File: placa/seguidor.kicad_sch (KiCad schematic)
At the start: 17 parts, among them J1 Conn_01x02_Pin, J2 Conn_01x15_Socket, SW1 btn_reset, SW2 btn_arranque, U1 ATmega328P-P, U2 LM7805_TO220, Y1 Crystal

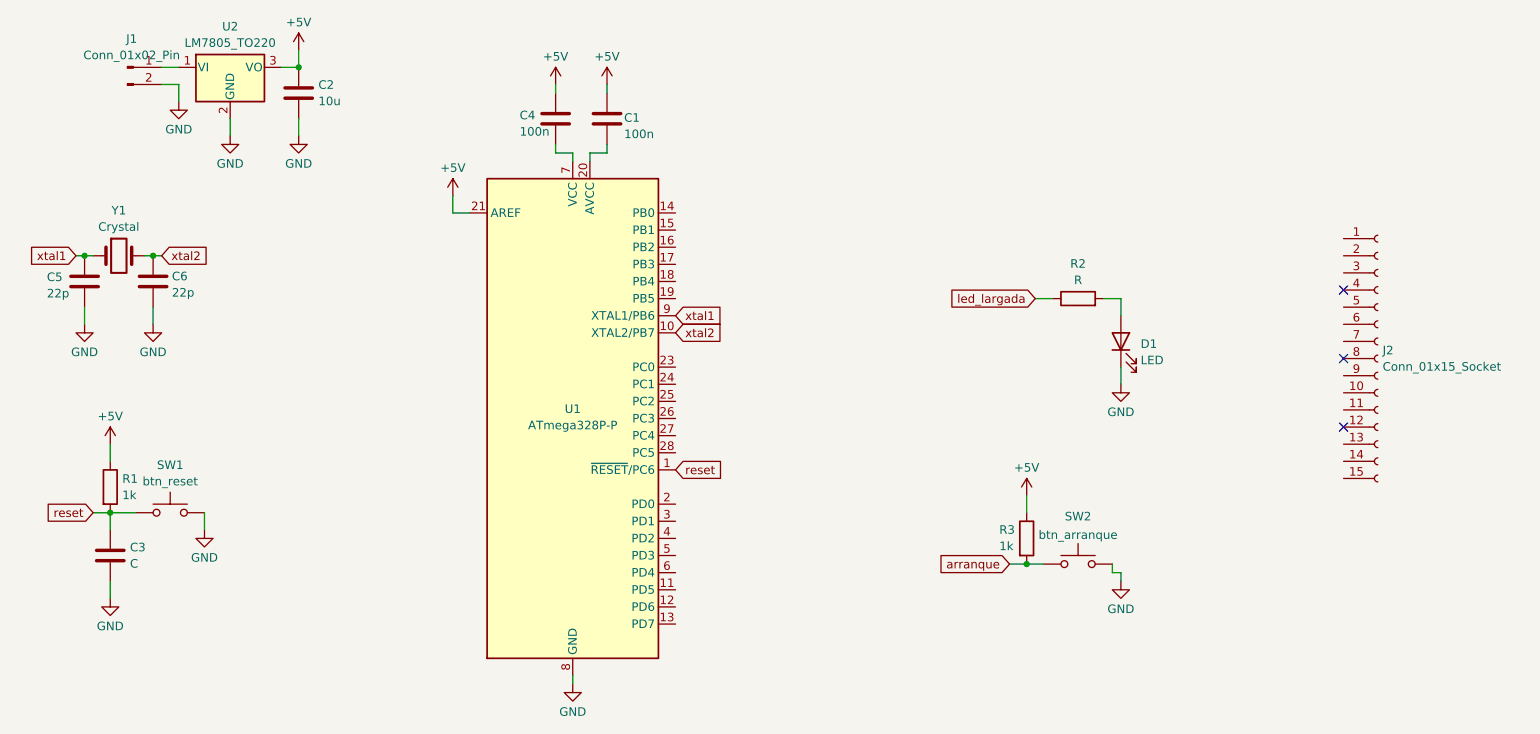
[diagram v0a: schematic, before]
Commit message: circuito modificado
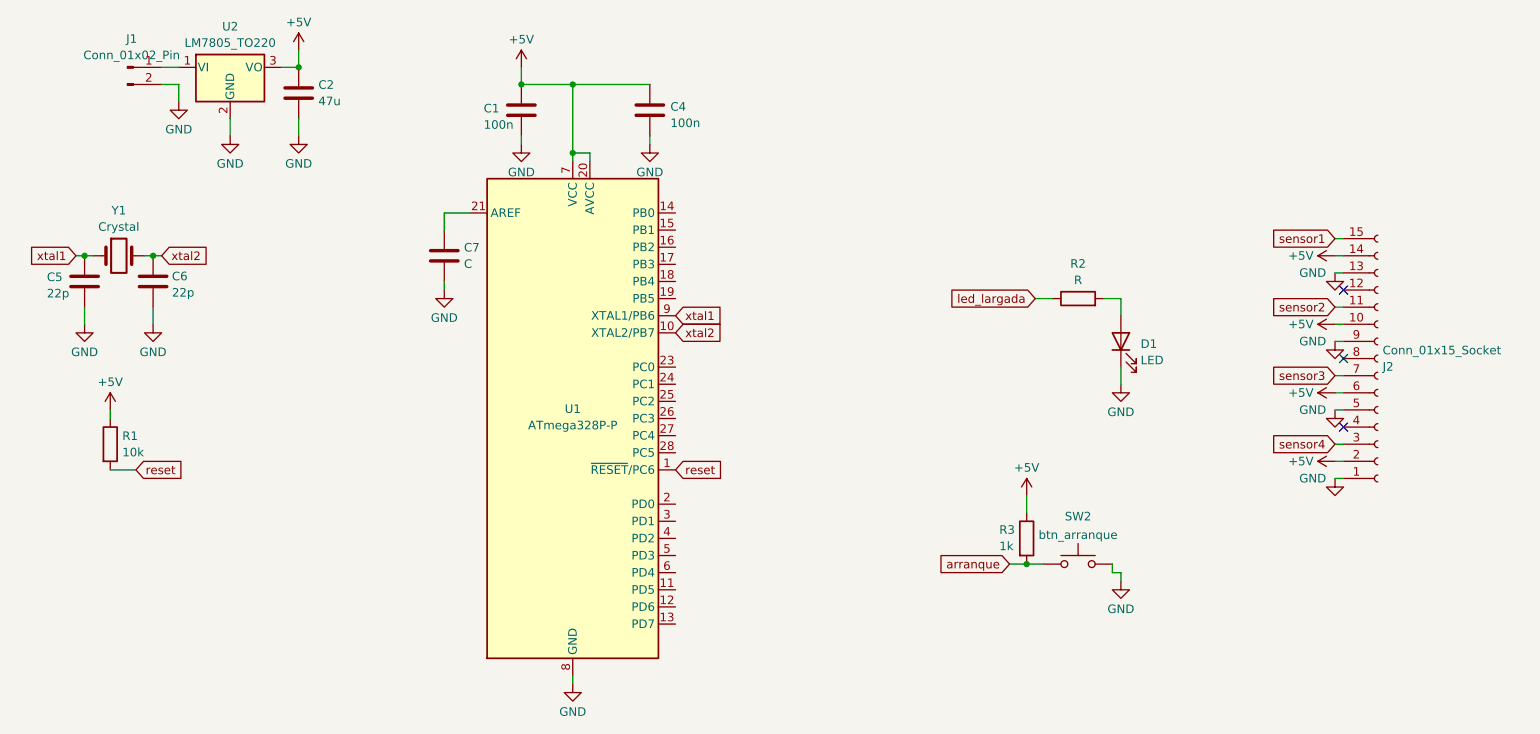
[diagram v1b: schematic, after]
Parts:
- removed C3: C, symbol Device:C
- removed SW1: btn_reset, symbol Switch:SW_Push
- added C7: C, symbol Device:C
- C1, C4: footprint (none) -> Capacitor_THT:C_Disc_D6.0mm_W2.5mm_P5.00mm
- C2: value 10u -> 47u; footprint (none) -> Capacitor_THT:CP_Radial_D5.0mm_P2.00mm
- C5, C6: footprint (none) -> Capacitor_THT:C_Disc_D5.0mm_W2.5mm_P5.00mm
- D1: footprint (none) -> LED_THT:LED_D4.0mm
- J2: footprint (none) -> Connector_PinSocket_2.54mm:PinSocket_1x15_P2.54mm_Horizontal
- R1: value 1k -> 10k
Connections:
- net +5V: now also J2.10 (Pin_10), J2.14 (Pin_14), J2.2 (Pin_2), J2.6 (Pin_6), U1.20 (AVCC), U1.7 (VCC); no longer U1.21 (AREF)
- net GND: now also C1.2, C4.2, J2.1 (Pin_1), J2.13 (Pin_13), J2.5 (Pin_5), J2.9 (Pin_9), C7.2
- net sensor2: now reaches J2.11 (Pin_11)
- net sensor1: now reaches J2.15 (Pin_15)
- net sensor4: now reaches J2.3 (Pin_3)
- net sensor3: now reaches J2.7 (Pin_7)
- new net: C7.1, U1.21 (AREF)
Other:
- moved on the sheet: C1, C4, R1
